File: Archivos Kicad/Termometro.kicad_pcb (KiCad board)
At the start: 2 copper layers, 53.3 x 66 mm, 24 parts, among them SW1 SW_Push, SW2 SW_Push, SW3 SW_Push, SW4 SW_Push, U1 LM358, U2 CC56-12EWA

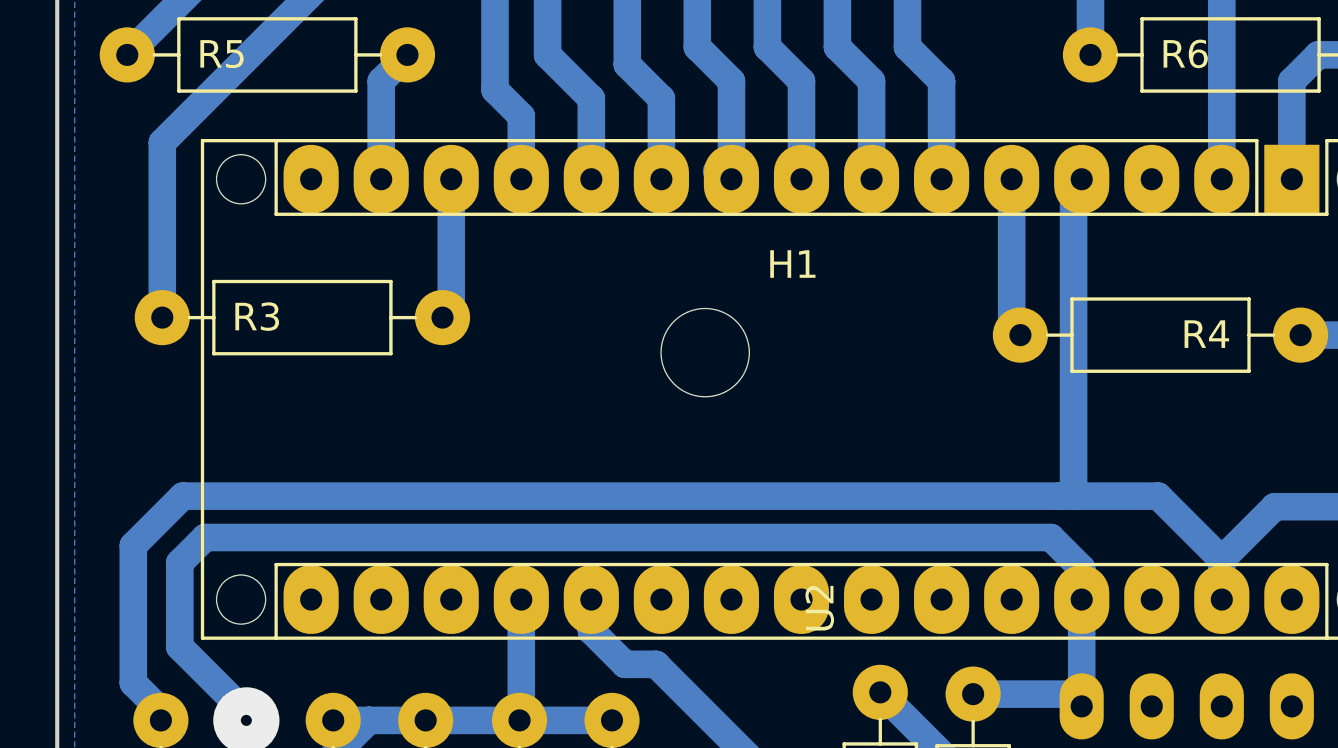
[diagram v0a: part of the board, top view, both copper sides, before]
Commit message: Docs-Datasheet/microentrenador-2021-v1.pdf
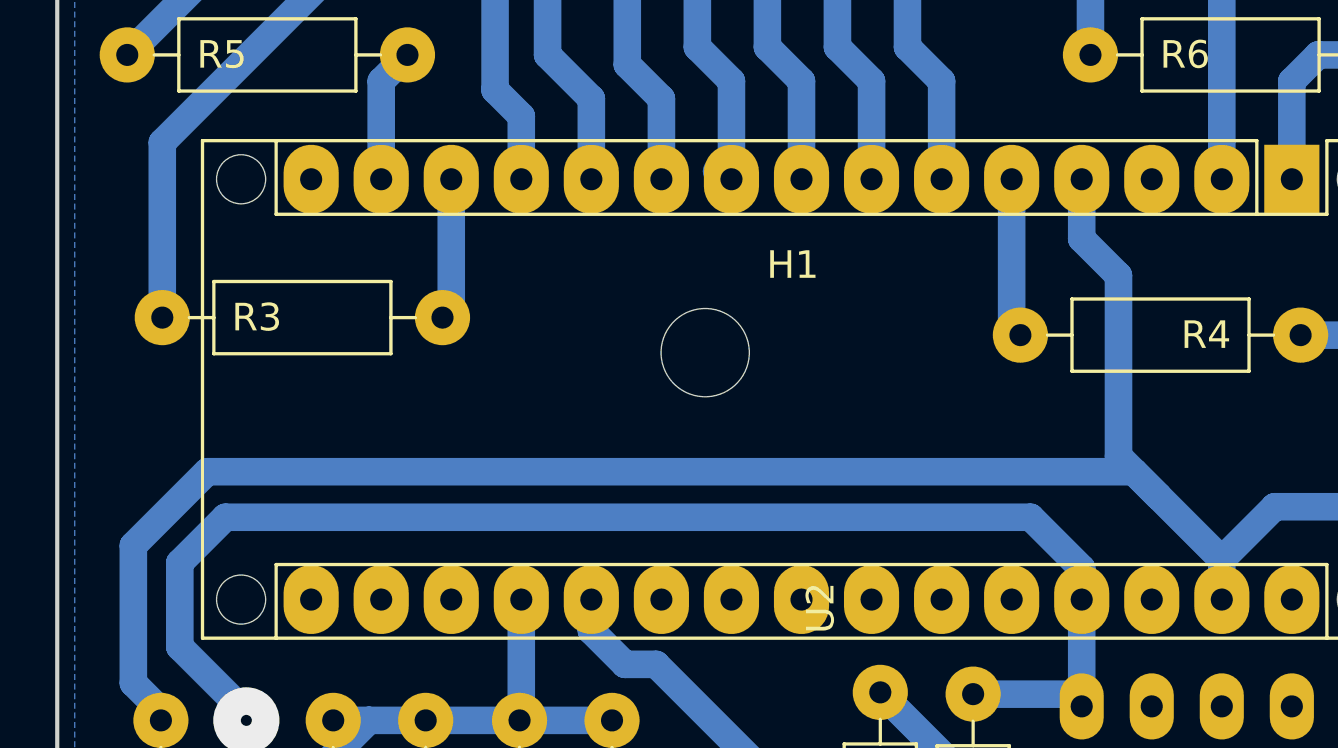
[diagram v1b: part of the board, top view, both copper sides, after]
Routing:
- net GND: track 101.3 -> 103.1 mm
- net +5V: track 103.6 -> 104.2 mm
